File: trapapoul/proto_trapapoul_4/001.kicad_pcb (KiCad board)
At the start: 2 copper layers, 110 x 50 mm, 116 parts, among them J101 HEADER_3x2, J401 HEADER_2, J402 HEADER_2, J403 HEADER_2, J410 HEADER_4, J730 HEADER_2, J801 HEADER_1, J802 HEADER_1, J901 HEADER_6, J902 HEADER_6, Q811 PBSS4320, Q812 PBSS5350, Q821 PBSS4320, Q822 PBSS5350, Q900 PBSS4320, U100 ATMEGA328P-A, U201 MCP7940, U500 MIC5205, U510 MIC5205, U520 MIC5205, U601 A3144, U602 A3144, U603 A3144, U604 A3144, U715 TLV431-DBZ, U830 MCP601-SOT, U900 PCF8574, X104 16M, X201 32.768K

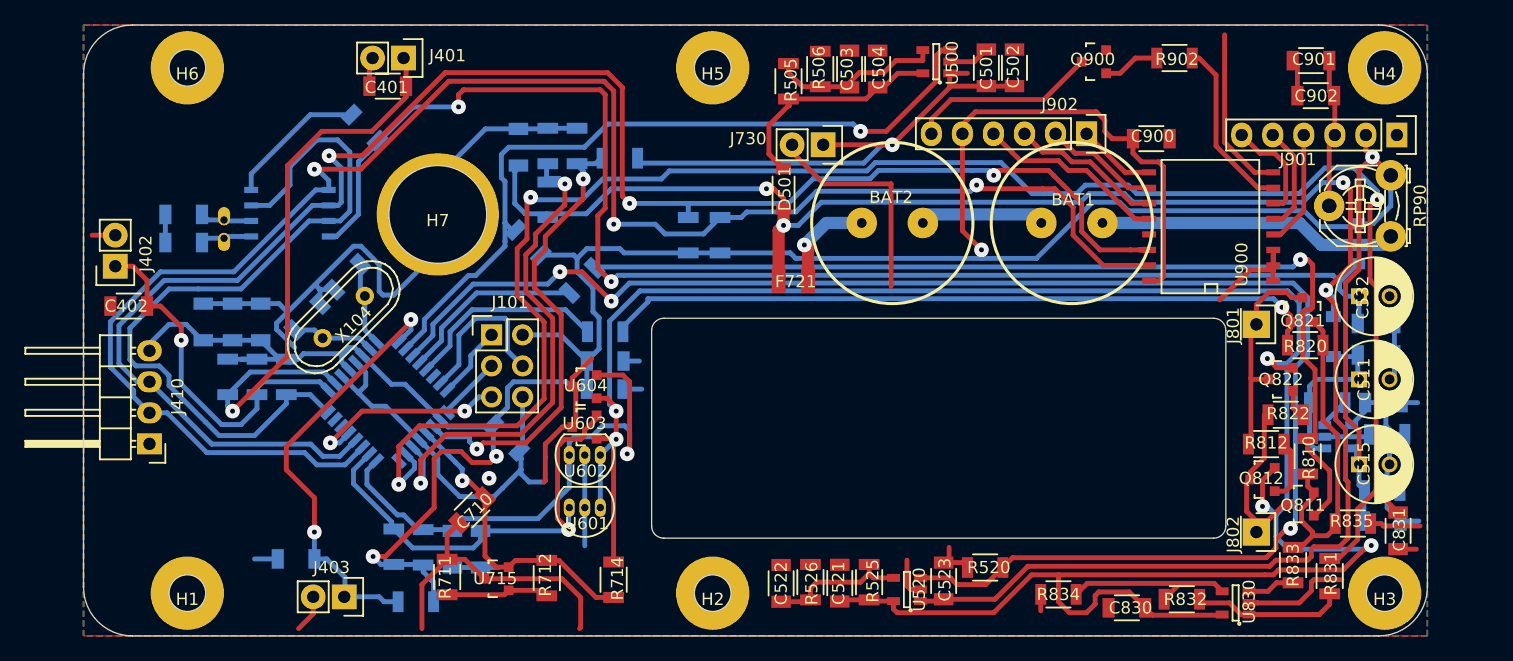
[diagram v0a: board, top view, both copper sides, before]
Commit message: prototrapapoul4 un peu retouché
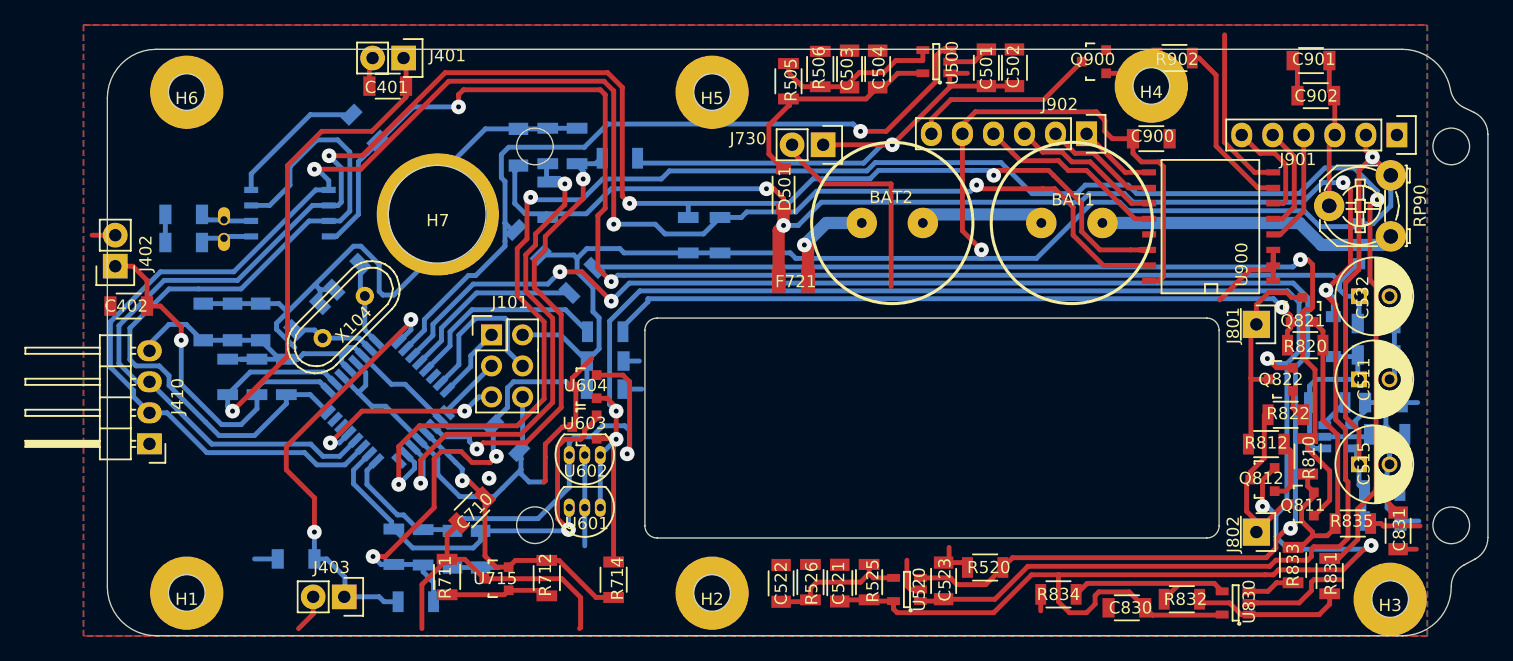
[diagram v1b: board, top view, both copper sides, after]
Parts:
- moved H4 19.2 mm to (187.4, 55.0)
- moved H5 2.00 mm to (151.4, 55.5)
- moved H6 2.00 mm to (108.5, 55.5)
- moved H3 0.67 mm to (206.9, 97.0)
- moved H2 0.05 mm to (151.4, 96.5)
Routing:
- net GND: vias 1 -> 0
- net (no net): vias 0 -> 1
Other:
- board size 110 x 50 mm -> 113 x 48 mm
